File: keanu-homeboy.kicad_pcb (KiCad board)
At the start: 2 copper layers, 32.9 x 50.4 mm, 15 parts, among them X1 Badgelife_sao_connector_v169b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

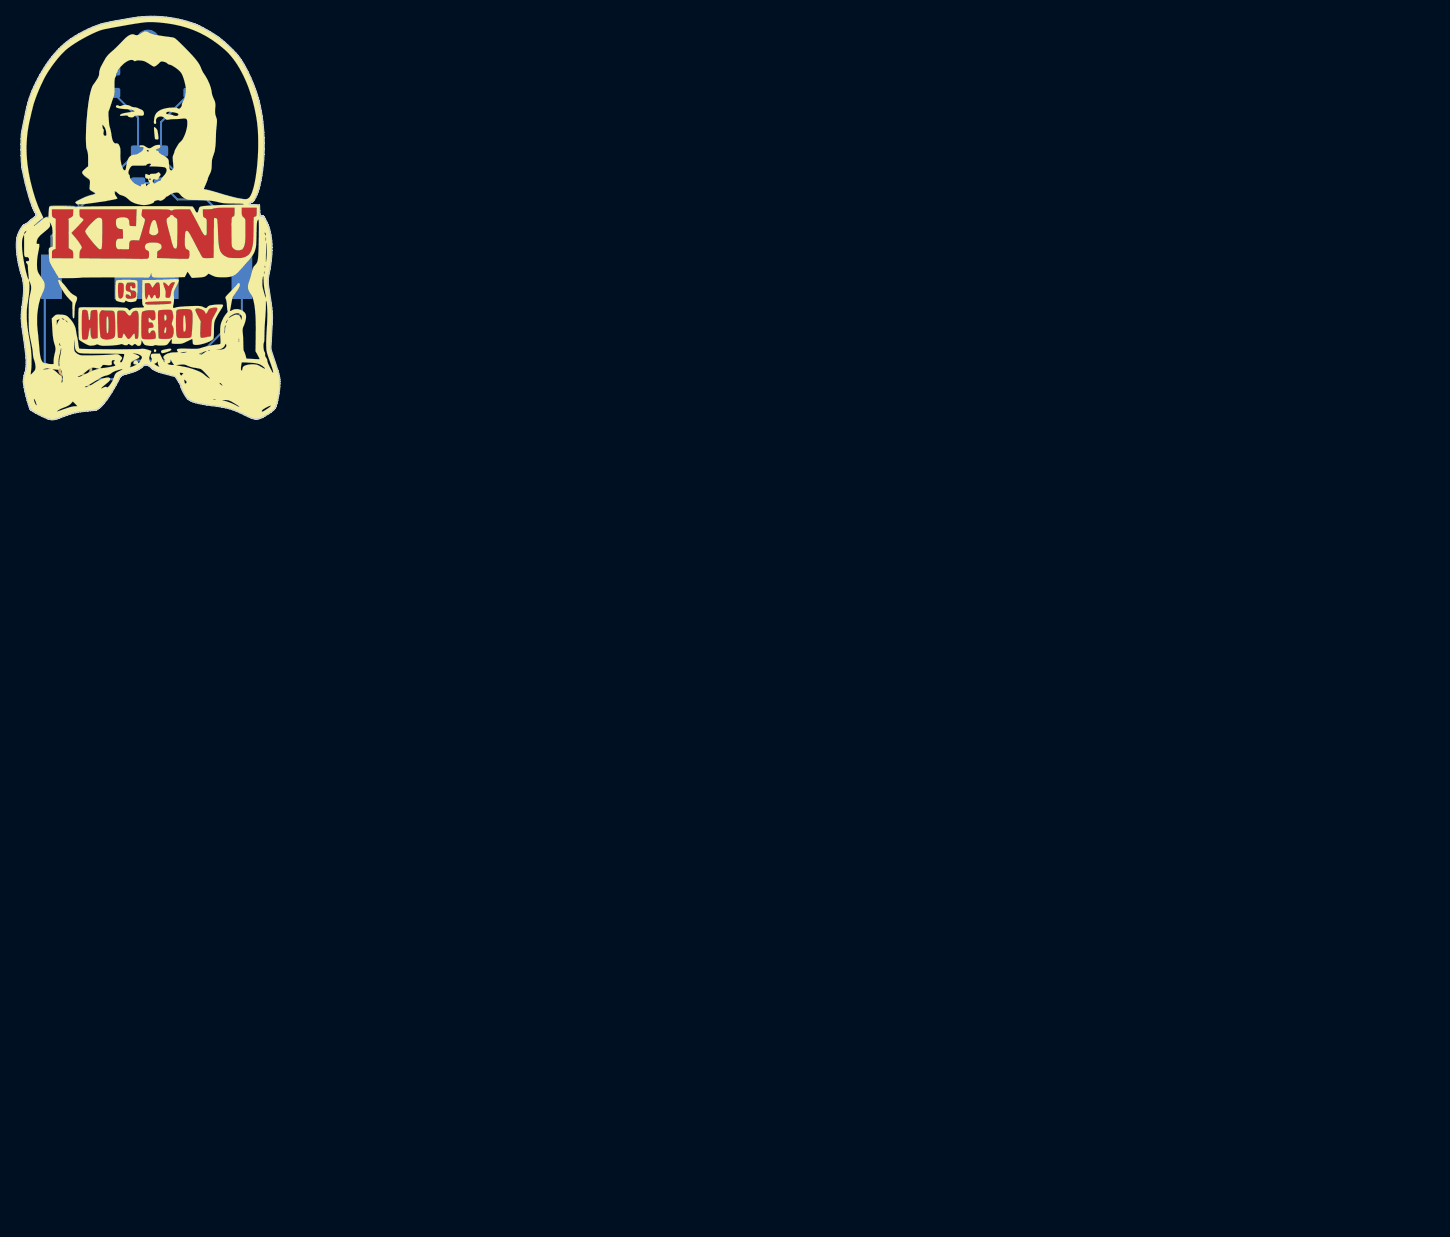
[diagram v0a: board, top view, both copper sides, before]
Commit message: updates for production
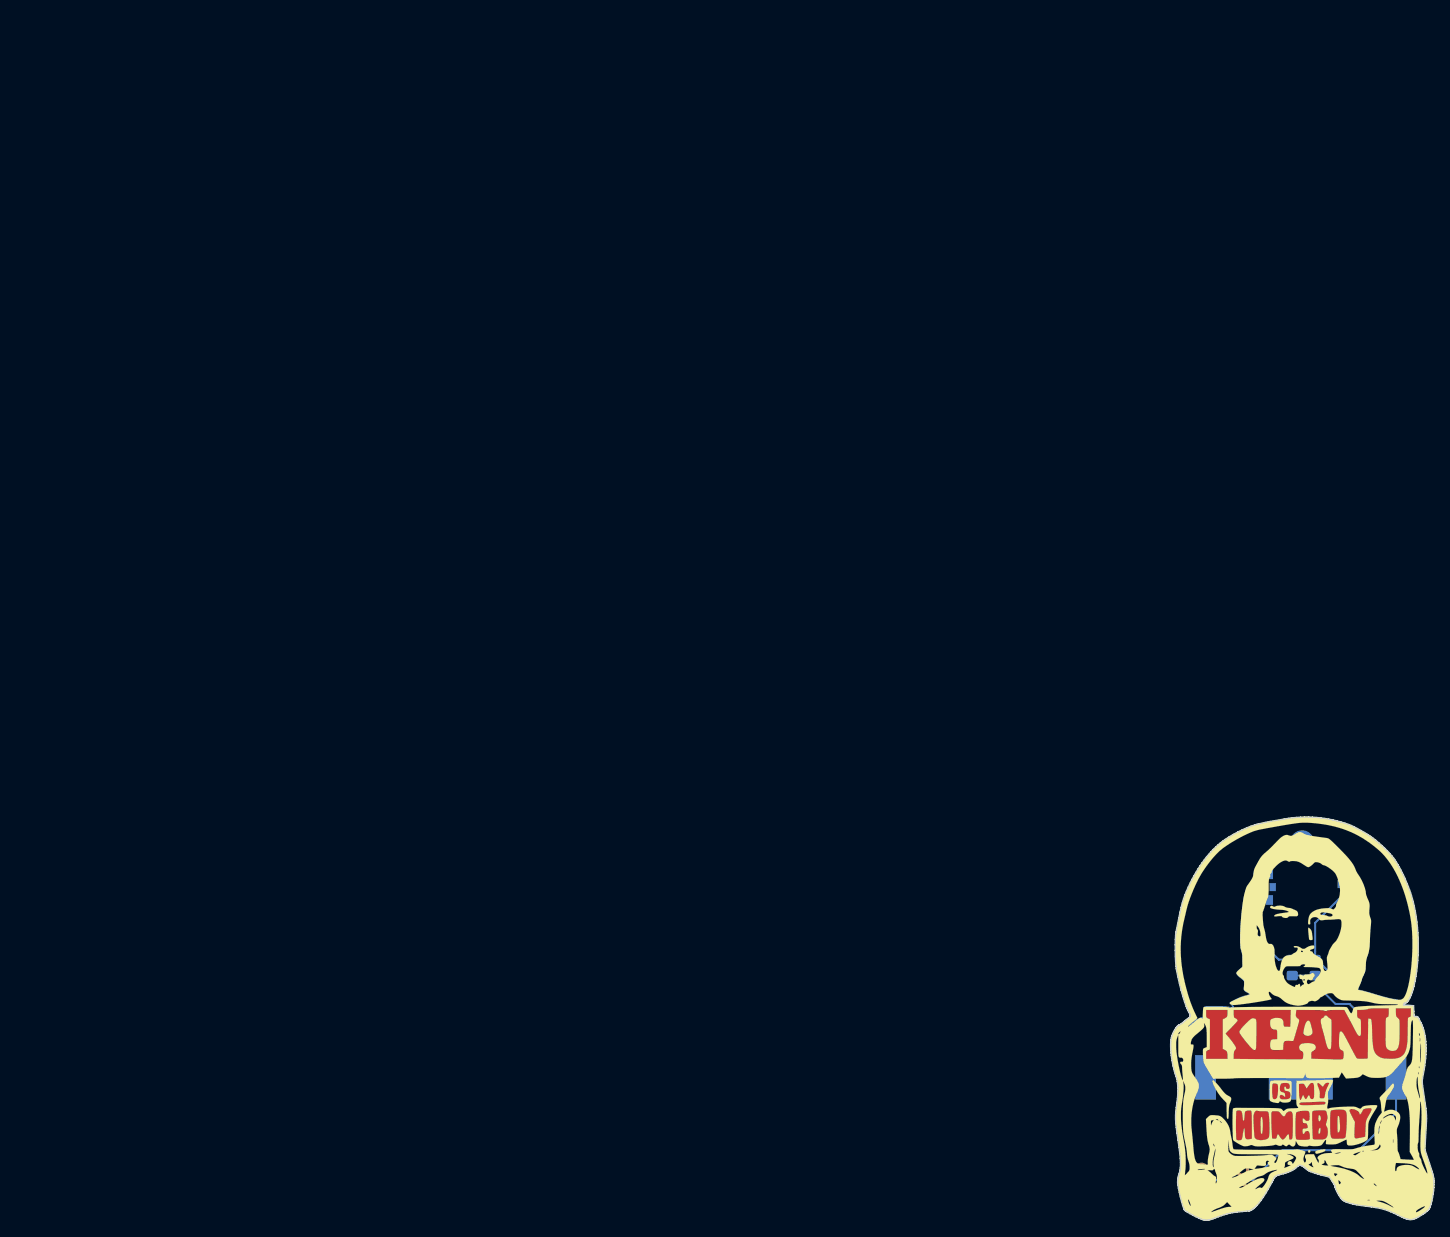
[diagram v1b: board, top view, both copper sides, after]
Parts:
- removed the G*** at (0.00, 0.00) (x6)
- added G*** (x6): LOGO, LOGO, F.Cu at (144.3, 100.1)
- D1, D2, D3, D4: footprint LED_SMD:LED_1206_3216Metric -> BadgePiratesFootprint:QBLP615
- R1, R2: footprint Resistor_SMD:R_1806_4516Metric -> Resistor_SMD:R_0805_2012Metric_Pad1.20x1.40mm_HandSolder
- X1: footprint my-ki-cad-parts:Badgelife-SAOv169-SAO-2x3 -> BadgePirateFootprints:Badgelife-SAOv169-SAO_Side_B.SLK
- moved D3 178.1 mm to (147.8, 78.2), turned to 90 degrees
- moved D4 177.8 mm to (148.1, 88.5), turned to 90 degrees
- moved ? 175.6 mm to (139.6, 73.0)
- moved BT1 175.6 mm to (139.5, 102.4)
- moved R1 175.6 mm to (138.4, 88.7)
- moved R2 175.6 mm to (141.2, 88.7)
- moved X1 175.6 mm to (129.2, 115.3)
- moved D2 173.7 mm to (132.5, 78.6)
- moved D1 172.6 mm to (131.1, 88.4)
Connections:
- X1 pad 3: Net-(X1-Pad3) -> unconnected-(X1-SDA-Pad3)
- X1 pad 4: Net-(X1-Pad4) -> unconnected-(X1-SCL-Pad4)
- X1 pad 5: Net-(X1-Pad5) -> unconnected-(X1-GPIO1-Pad5)
- X1 pad 6: Net-(X1-Pad6) -> unconnected-(X1-GPIO2-Pad6)
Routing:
- net /VDD: track 86.7 -> 56.5 mm
- net Net-(D1-A): track 13.9 -> 15.7 mm
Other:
- net class Default removed
